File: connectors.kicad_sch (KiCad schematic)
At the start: 4 parts, among them J1 Conn_01x05, J2 Conn_01x07, J4 Conn_01x07, J5 Conn_01x02

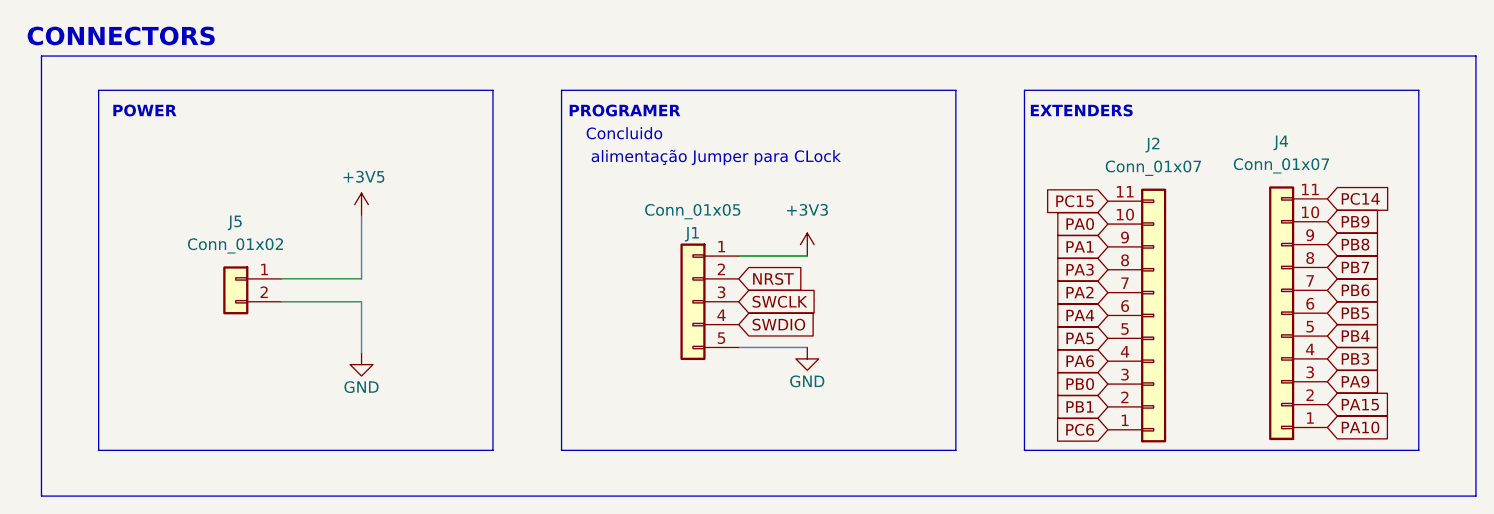
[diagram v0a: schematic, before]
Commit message: [feat] PCB routing
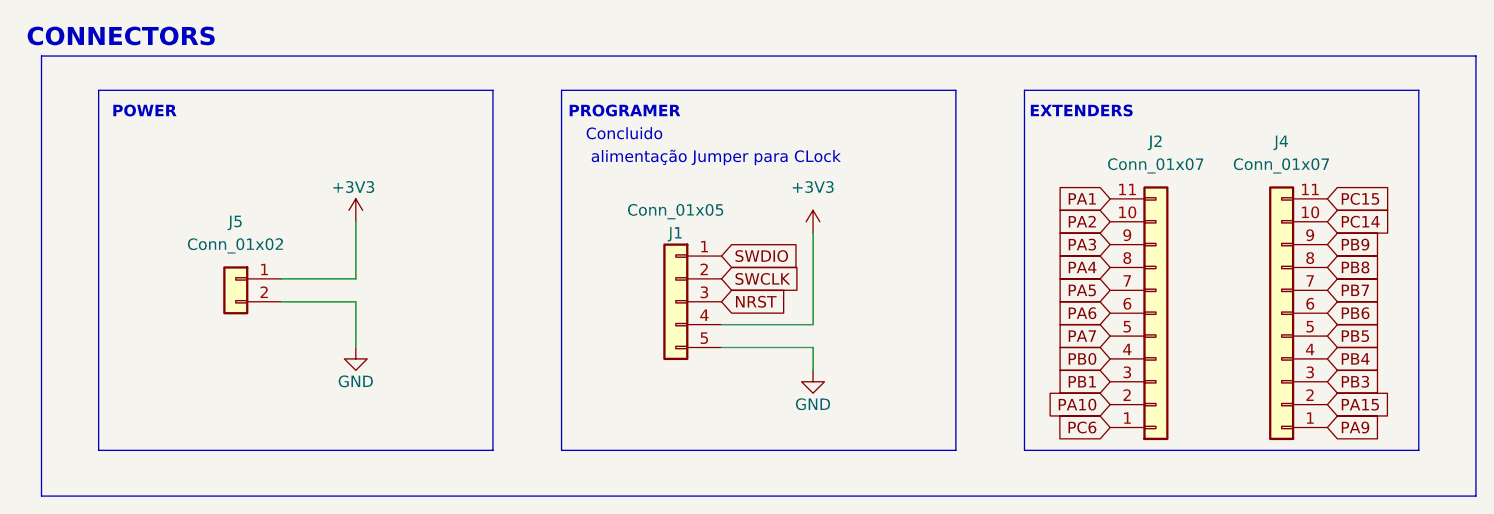
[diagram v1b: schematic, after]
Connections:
- net +3V5 is gone; now on net +3V3: J5.1 (Pin_1)
- net PA0 is gone; now on net PA2: J2.10 (Pin_10)
- net +3V3: now also J1.4 (Pin_4); no longer J1.1 (Pin_1)
- net NRST: now also J1.3 (Pin_3); no longer J1.2 (Pin_2)
- net PA1: now also J2.11 (Pin_11); no longer J2.9 (Pin_9)
- net PA10: now also J2.2 (Pin_2); no longer J4.1 (Pin_1)
- net PA2: no longer J2.7 (Pin_7)
- net PA3: now also J2.9 (Pin_9); no longer J2.8 (Pin_8)
- net PA4: now also J2.8 (Pin_8); no longer J2.6 (Pin_6)
- net PA5: now also J2.7 (Pin_7); no longer J2.5 (Pin_5)
- net PA6: now also J2.6 (Pin_6); no longer J2.4 (Pin_4)
- net PA9: now also J4.1 (Pin_1); no longer J4.3 (Pin_3)
- net PB0: now also J2.4 (Pin_4); no longer J2.3 (Pin_3)
- net PB1: now also J2.3 (Pin_3); no longer J2.2 (Pin_2)
- net PB3: now also J4.3 (Pin_3); no longer J4.4 (Pin_4)
- net PB4: now also J4.4 (Pin_4); no longer J4.5 (Pin_5)
- net PB5: now also J4.5 (Pin_5); no longer J4.6 (Pin_6)
- net PB6: now also J4.6 (Pin_6); no longer J4.7 (Pin_7)
- net PB7: now also J4.7 (Pin_7); no longer J4.8 (Pin_8)
- net PB8: now also J4.8 (Pin_8); no longer J4.9 (Pin_9)
- net PB9: now also J4.9 (Pin_9); no longer J4.10 (Pin_10)
- net PC14: now also J4.10 (Pin_10); no longer J4.11 (Pin_11)
- net PC15: now also J4.11 (Pin_11); no longer J2.11 (Pin_11)
- net SWCLK: now also J1.2 (Pin_2); no longer J1.3 (Pin_3)
- net SWDIO: now also J1.1 (Pin_1); no longer J1.4 (Pin_4)
- new net PA7: J2.5 (Pin_5)
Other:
- moved on the sheet: J1

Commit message: Modifying footprint positions
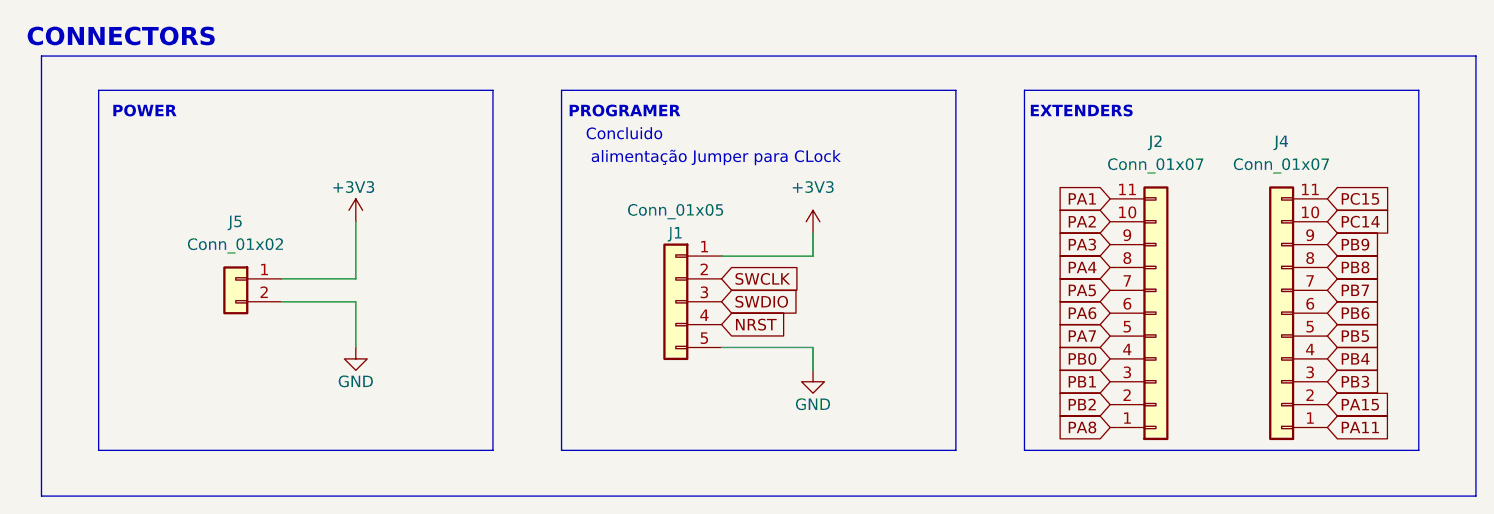
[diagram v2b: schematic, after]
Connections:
- net +3V3: now also J1.1 (Pin_1); no longer J1.4 (Pin_4)
- net NRST: now also J1.4 (Pin_4); no longer J1.3 (Pin_3)
- net SWDIO: now also J1.3 (Pin_3); no longer J1.1 (Pin_1)
- net PA10 renamed PB2
- net PA9 renamed PA11
- net PC6 renamed PA8
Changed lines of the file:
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@@
+		)
+	)
+	(bus
+		(pts
+			(xy 69.215 74.295) (xy 69.215 123.19)
+		)
+		(stroke
+			(width 0)
+			(type default)
 		)
 	)
 	(wire
 		(pts
-			(xy 154.94 104.14) (xy 144.78 104.14)
-		)
-		(stroke
-			(width 0)
-			(type default)
-		)
-	)
-	(bus
-		(pts
-			(xy 69.215 74.295) (xy 69.215 123.19)
+			(xy 154.94 109.22) (xy 154.94 106.68)
 		)
 		(stroke
@@
 	(wire
 		(pts
-			(xy 154.94 109.22) (xy 154.94 106.68)
+			(xy 154.94 96.52) (xy 154.94 93.98)
 		)
 		(stroke
@@
 		)
 	)
+	(wire
+		(pts
+			(xy 144.78 96.52) (xy 154.94 96.52)
+		)
+		(stroke
+			(width 0)
+			(type default)
+		)
+	)
 	(bus
 		(pts
@@
 			(width 0)
 			(type dot)
-		)
-	)
-	(wire
-		(pts
-			(xy 154.94 93.98) (xy 154.94 104.14)
-		)
-		(stroke
-			(width 0)
-			(type default)
 		)
 	)
@@
 		)
 	)
-	(global_label "PC6"
+	(global_label "PA8"
 		(shape input)
 		(at 187.96 115.57 180)
@@
 		)
 		(property "Intersheetrefs" "${INTERSHEET_REFS}"
-			(at 181.2253 115.57 0)
-			(effects
-				(font
-					(size 1.27 1.27)
-				)
-				(justify right)
-				(hide yes)
-			)
-		)
-	)
-	(global_label "PA9"
+			(at 181.4067 115.57 0)
+			(effects
+				(font
+					(size 1.27 1.27)
+				)
+				(justify right)
+				(hide yes)
+			)
+		)
+	)
+	(global_label "SWDIO"
+		(shape input)
+		(at 144.78 101.6 0)
+		(fields_autoplaced yes)
+		(effects
+			(font
+				(size 1.27 1.27)
+			)
+			(justify left)
+		)
+		(property "Intersheetrefs" "${INTERSHEET_REFS}"
+			(at 153.6314 101.6 0)
+			(effects
+				(font
+					(size 1.27 1.27)
+				)
+				(justify left)
+				(hide yes)
+			)
+		)
+	)
+	(global_label "PA15"
+		(shape input)
+		(at 212.09 113.03 0)
+		(fields_autoplaced yes)
+		(effects
+			(font
+				(size 1.27 1.27)
+			)
+			(justify left)
+		)
+		(property "Intersheetrefs" "${INTERSHEET_REFS}"
+			(at 219.8528 113.03 0)
+			(effects
+				(font
+					(size 1.27 1.27)
+				)
+				(justify left)
+				(hide yes)
+			)
+		)
+	)
+	(global_label "NRST"
+		(shape input)
+		(at 144.78 104.14 0)
+		(fields_autoplaced yes)
+		(effects
+			(font
+				(size 1.27 1.27)
+			)
+			(justify left)
+		)
+		(property "Intersheetrefs" "${INTERSHEET_REFS}"
+			(at 152.5428 104.14 0)
+			(effects
+				(font
+					(size 1.27 1.27)
+				)
+				(justify left)
+				(hide yes)
+			)
+		)
+	)
+	(global_label "PA11"
 		(shape input)
 		(at 212.09 115.57 0)
@@
 		)
 		(property "Intersheetrefs" "${INTERSHEET_REFS}"
-			(at 218.6433 115.57 0)
-			(effects
-				(font
-					(size 1.27 1.27)
-				)
-				(justify left)
-				(hide yes)
-			)
-		)
-	)
-	(global_label "SWDIO"
-		(shape input)
-		(at 144.78 96.52 0)
-		(fields_autoplaced yes)
-		(effects
-			(font
-				(size 1.27 1.27)
-			)
-			(justify left)
-		)
-		(property "Intersheetrefs" "${INTERSHEET_REFS}"
-			(at 153.6314 96.52 0)
-			(effects
-				(font
-					(size 1.27 1.27)
-				)
-				(justify left)
-				(hide yes)
-			)
-		)
-	)
-	(global_label "PA15"
-		(shape input)
-		(at 212.09 113.03 0)
-		(fields_autoplaced yes)
-		(effects
-			(font
-				(size 1.27 1.27)
-			)
-			(justify left)
-		)
-		(property "Intersheetrefs" "${INTERSHEET_REFS}"
-			(at 219.8528 113.03 0)
-			(effects
-				(font
-					(size 1.27 1.27)
-				)
-				(justify left)
-				(hide yes)
-			)
-		)
-	)
-	(global_label "NRST"
-		(shape input)
-		(at 144.78 101.6 0)
-		(fields_autoplaced yes)
-		(effects
-			(font
-				(size 1.27 1.27)
-			)
-			(justify left)
-		)
-		(property "Intersheetrefs" "${INTERSHEET_REFS}"
-			(at 152.5428 101.6 0)
-			(effects
-				(font
-					(size 1.27 1.27)
-				)
-				(justify left)
-				(hide yes)
-			)
-		)
-	)
-	(global_label "PA10"
+			(at 219.8528 115.57 0)
+			(effects
+				(font
+					(size 1.27 1.27)
+				)
+				(justify left)
+				(hide yes)
+			)
+		)
+	)
+	(global_label "PA4"
+		(shape input)
+		(at 187.96 97.79 180)
+		(fields_autoplaced yes)
+		(effects
+			(font
+				(size 1.27 1.27)
+			)
+			(justify right)
+		)
+		(property "Intersheetrefs" "${INTERSHEET_REFS}"
+			(at 181.4067 97.79 0)
+			(effects
+				(font
+					(size 1.27 1.27)
+				)
+				(justify right)
+				(hide yes)
+			)
+		)
+	)
+	(global_label "SWCLK"
+		(shape input)
+		(at 144.78 99.06 0)
+		(fields_autoplaced yes)
+		(effects
+			(font
+				(size 1.27 1.27)
+			)
+			(justify left)
+		)
+		(property "Intersheetrefs" "${INTERSHEET_REFS}"
+			(at 153.9942 99.06 0)
+			(effects
+				(font
+					(size 1.27 1.27)
+				)
+				(justify left)
+				(hide yes)
+			)
+		)
+	)
+	(global_label "PC14"
+		(shape input)
+		(at 212.09 92.71 0)
+		(fields_autoplaced yes)
+		(effects
+			(font
+				(size 1.27 1.27)
+			)
+			(justify left)
+		)
+		(property "Intersheetrefs" "${INTERSHEET_REFS}"
+			(at 220.0342 92.71 0)
+			(effects
+				(font
+					(size 1.27 1.27)
+				)
+				(justify left)
+				(hide yes)
+			)
+		)
+	)
+	(global_label "PB2"
 		(shape input)
 		(at 187.96 113.03 180)
@@
 		)
 		(property "Intersheetrefs" "${INTERSHEET_REFS}"
-			(at 180.1972 113.03 0)
-			(effects
-				(font
-					(size 1.27 1.27)
-				)
-				(justify right)
-				(hide yes)
-			)
-		)
-	)
-	(global_label "PA4"
-		(shape input)
-		(at 187.96 97.79 180)
-		(fields_autoplaced yes)
-		(effects
-			(font
-				(size 1.27 1.27)
-			)
-			(justify right)
-		)
-		(property "Intersheetrefs" "${INTERSHEET_REFS}"
-			(at 181.4067 97.79 0)
-			(effects
-				(font
-					(size 1.27 1.27)
-				)
-				(justify right)
-				(hide yes)
-			)
-		)
-	)
-	(global_label "SWCLK"
-		(shape input)
-		(at 144.78 99.06 0)
-		(fields_autoplaced yes)
-		(effects
-			(font
-				(size 1.27 1.27)
-			)
-			(justify left)
-		)
-		(property "Intersheetrefs" "${INTERSHEET_REFS}"
-			(at 153.9942 99.06 0)
-			(effects
-				(font
-					(size 1.27 1.27)
-				)
-				(justify left)
-				(hide yes)
-			)
-		)
-	)
-	(global_label "PC14"
-		(shape input)
-		(at 212.09 92.71 0)
-		(fields_autoplaced yes)
-		(effects
-			(font
-				(size 1.27 1.27)
-			)
-			(justify left)
-		)
-		(property "Intersheetrefs" "${INTERSHEET_REFS}"
-			(at 220.0342 92.71 0)
-			(effects
-				(font
-					(size 1.27 1.27)
-				)
-				(justify left)
-				(hide yes)
-			)
+			(at 181.2253 113.03 0)
+			(effects
+				(font
+					(size 1.27 1.27)
+				)
+				(justify right)
+				(hide yes)
+			)
